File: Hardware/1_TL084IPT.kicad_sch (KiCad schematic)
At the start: 23 parts, among them J7 Screw_Terminal_01x08, Q1 N_Mosfet, Q2 N_Mosfet, Q20 N_Mosfet, Q3 N_Mosfet, U11 TL084

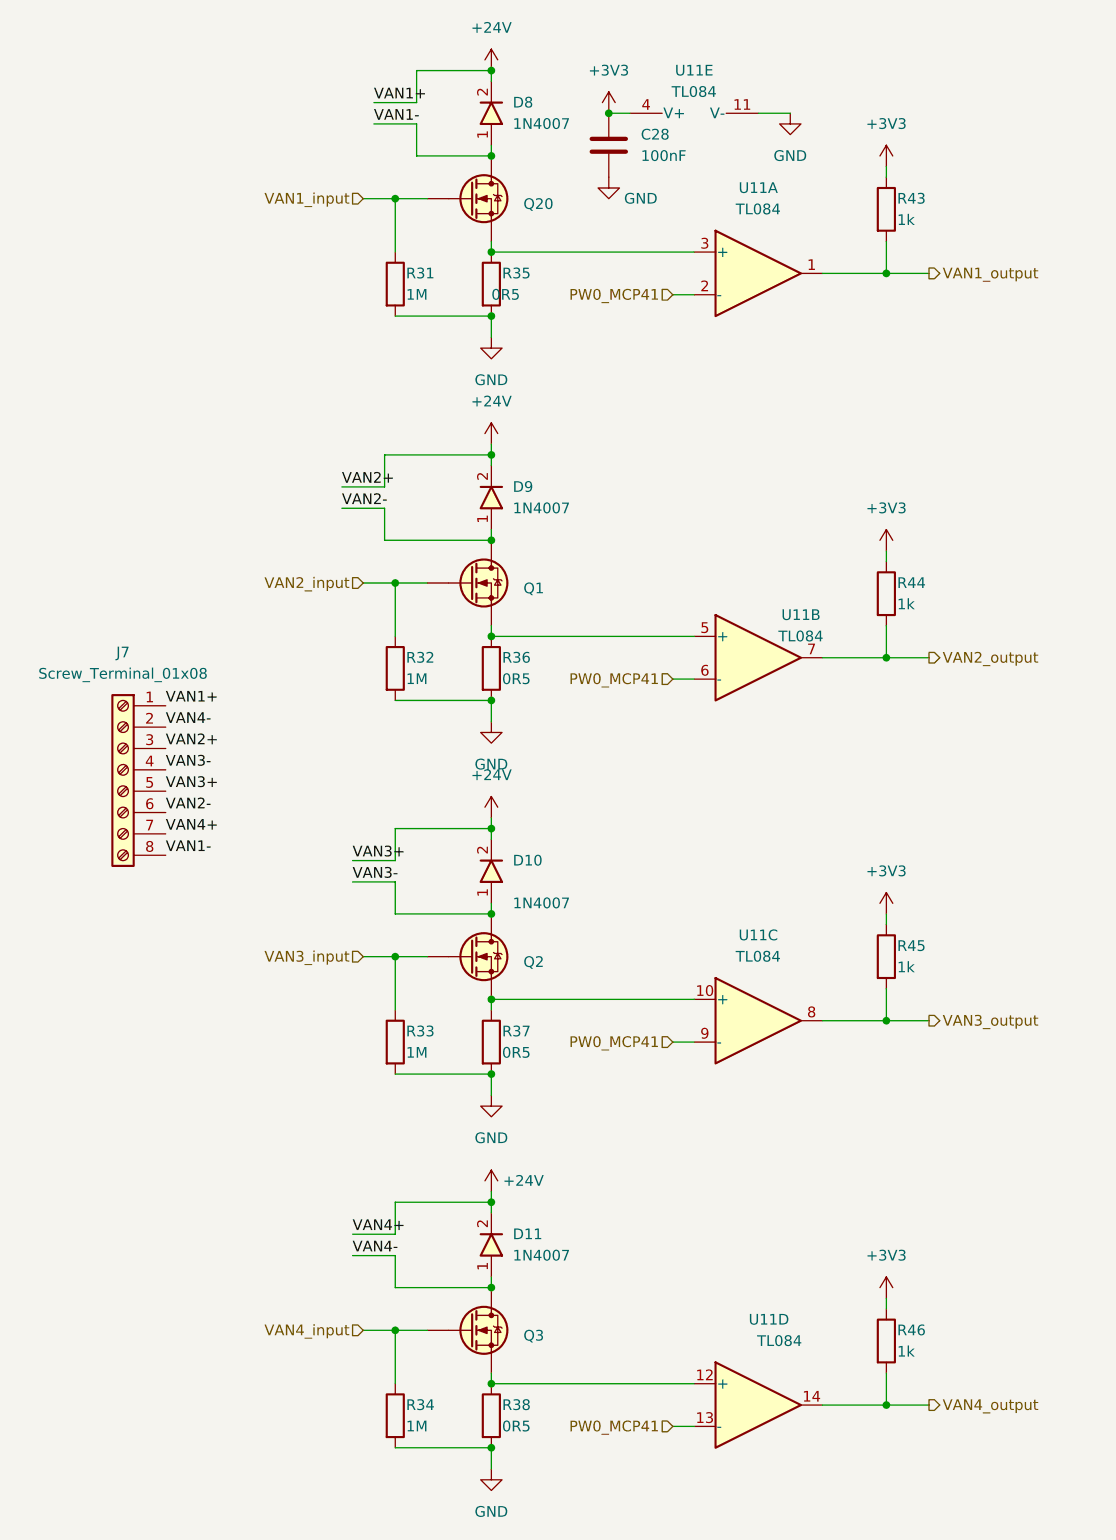
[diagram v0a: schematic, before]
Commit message: layout part 2
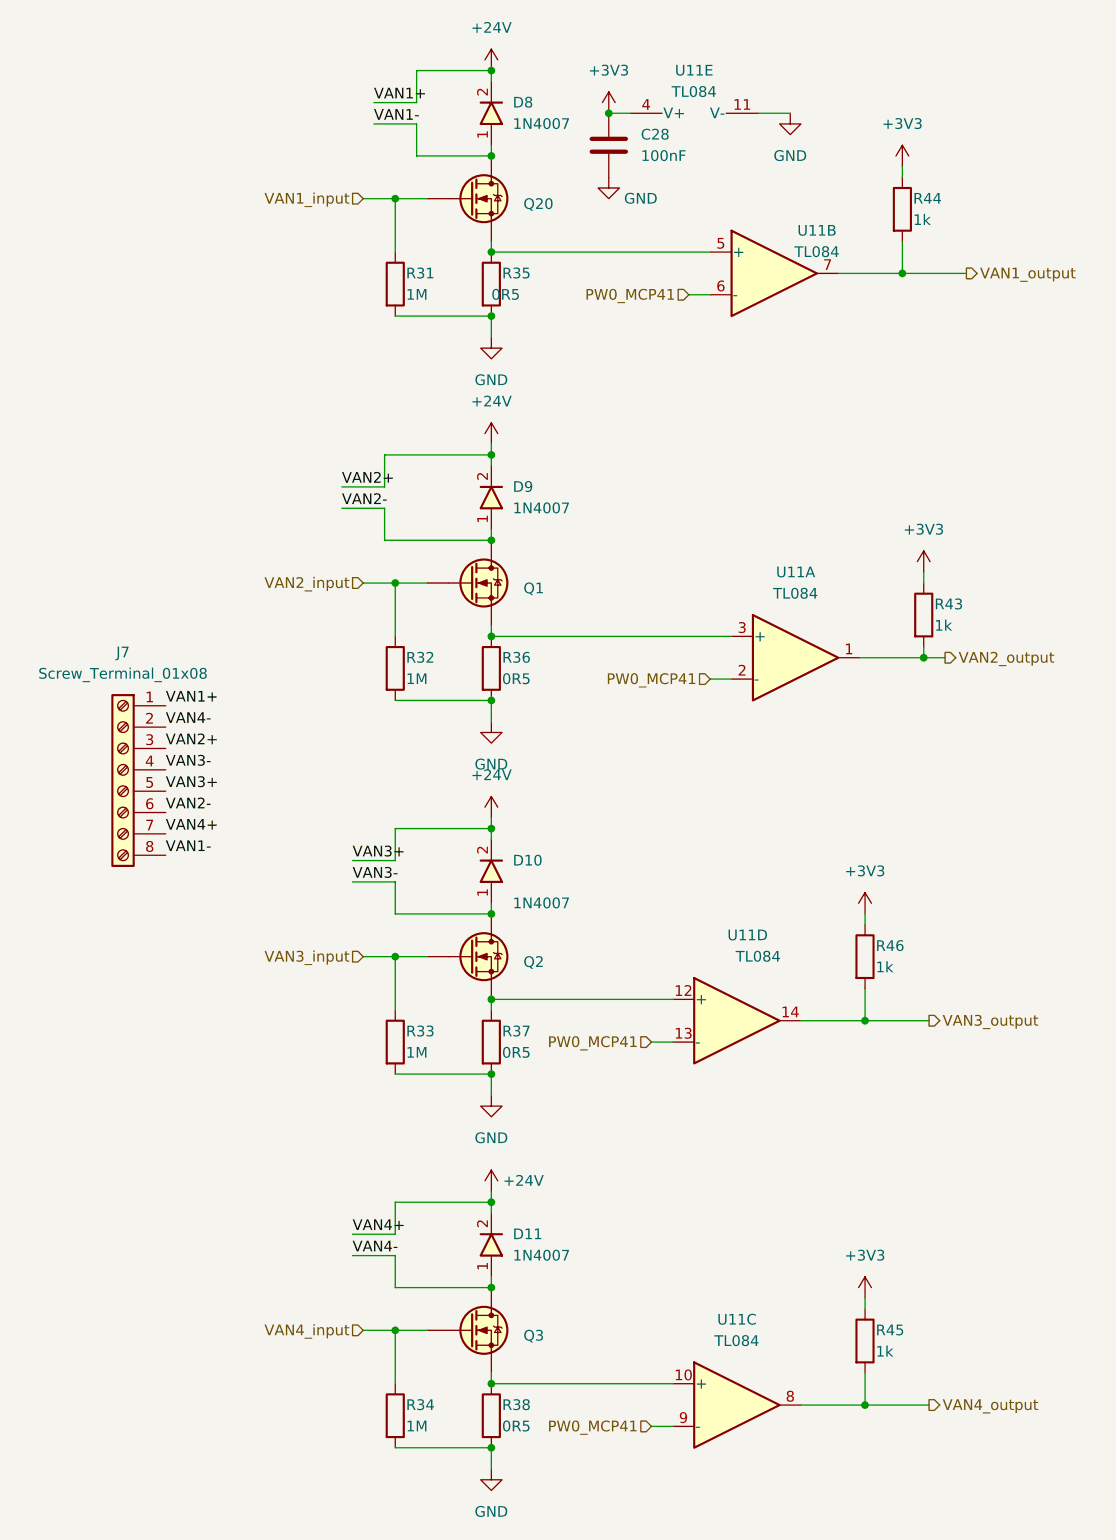
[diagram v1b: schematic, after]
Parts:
- D10, D11, D8, D9: footprint IVS_FOOTPRINTS:D_MiniMELF -> IVS_FOOTPRINTS:D_SOD323
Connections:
- net VAN1_output: now also R44.2, U11.7; no longer R43.2, U11.1
- net VAN2_output: now also R43.2, U11.1; no longer R44.2, U11.7
- net VAN3_output: now also R46.2, U11.14; no longer R45.2, U11.8
- net VAN4_output: now also R45.2, U11.8; no longer R46.2, U11.14
- net at Q20.2 (S), R35.1: now also U11.5 (+); no longer U11.3 (+)
- net at Q2.2 (S), R37.1: now also U11.12 (+); no longer U11.10 (+)
- net at Q3.2 (S), R38.1: now also U11.10 (+); no longer U11.12 (+)
- net at Q1.2 (S), R36.1: now also U11.3 (+); no longer U11.5 (+)
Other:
- moved on the sheet: R43, R44, R45, R46, U11A, U11B, U11C, U11D
